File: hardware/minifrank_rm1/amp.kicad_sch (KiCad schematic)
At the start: 20 parts, among them U5 LM358

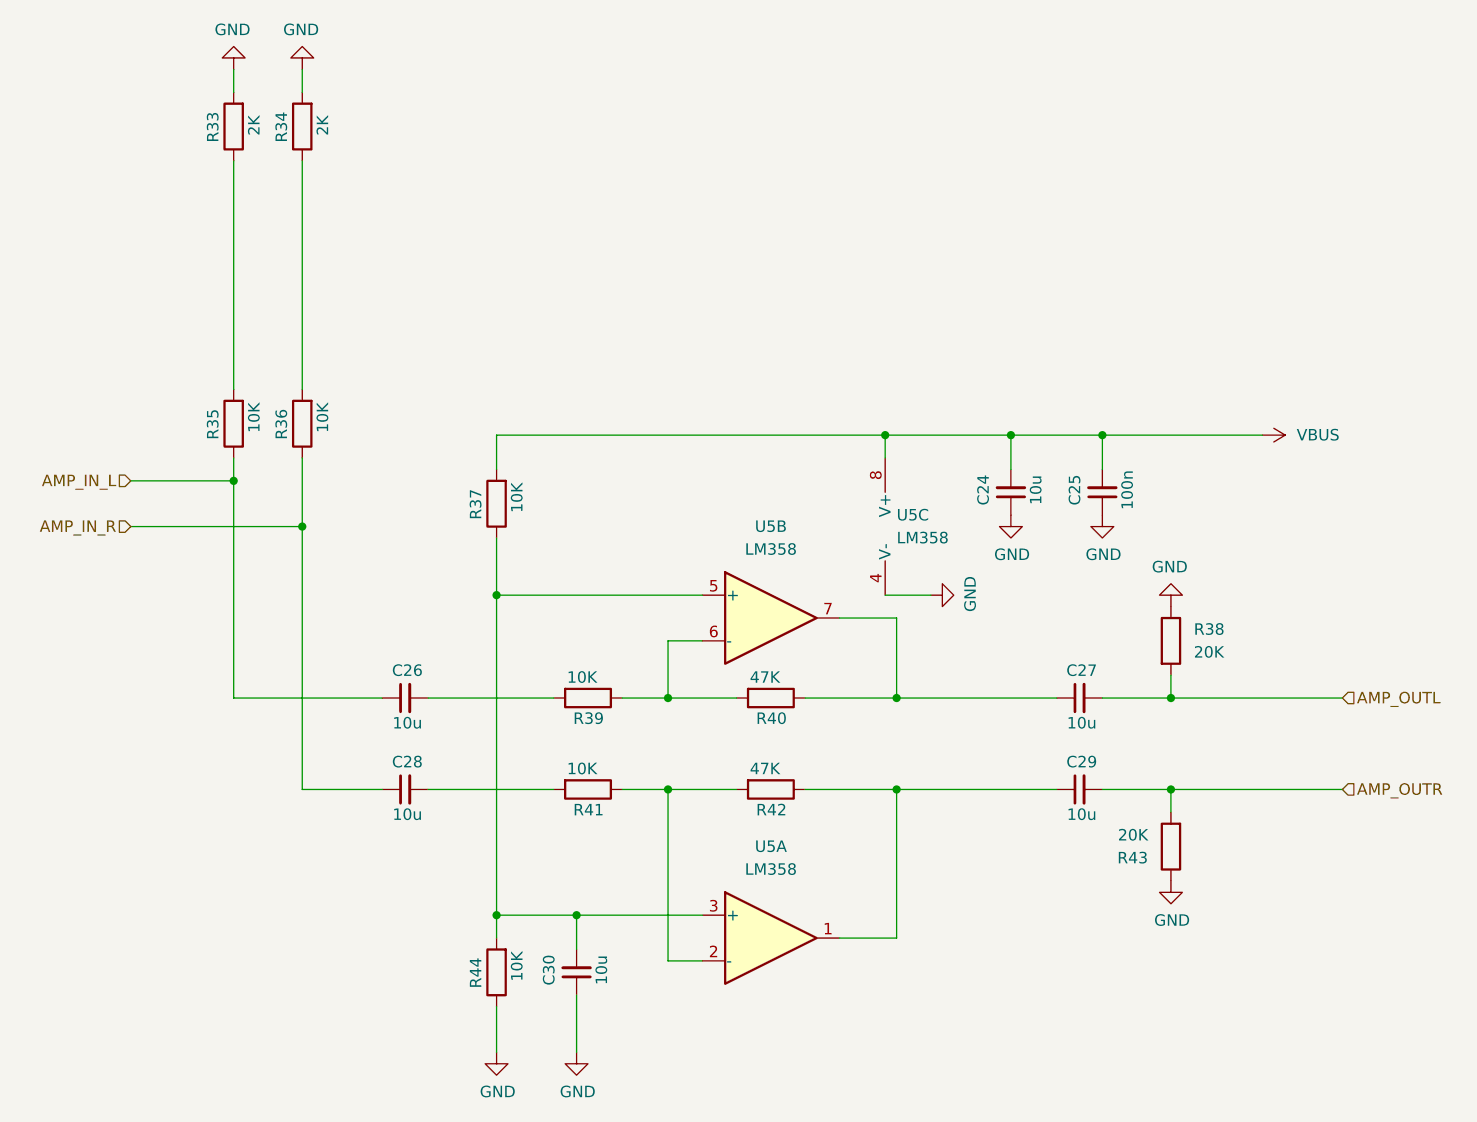
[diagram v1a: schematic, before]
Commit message: MiniFRANK 2.05 Release
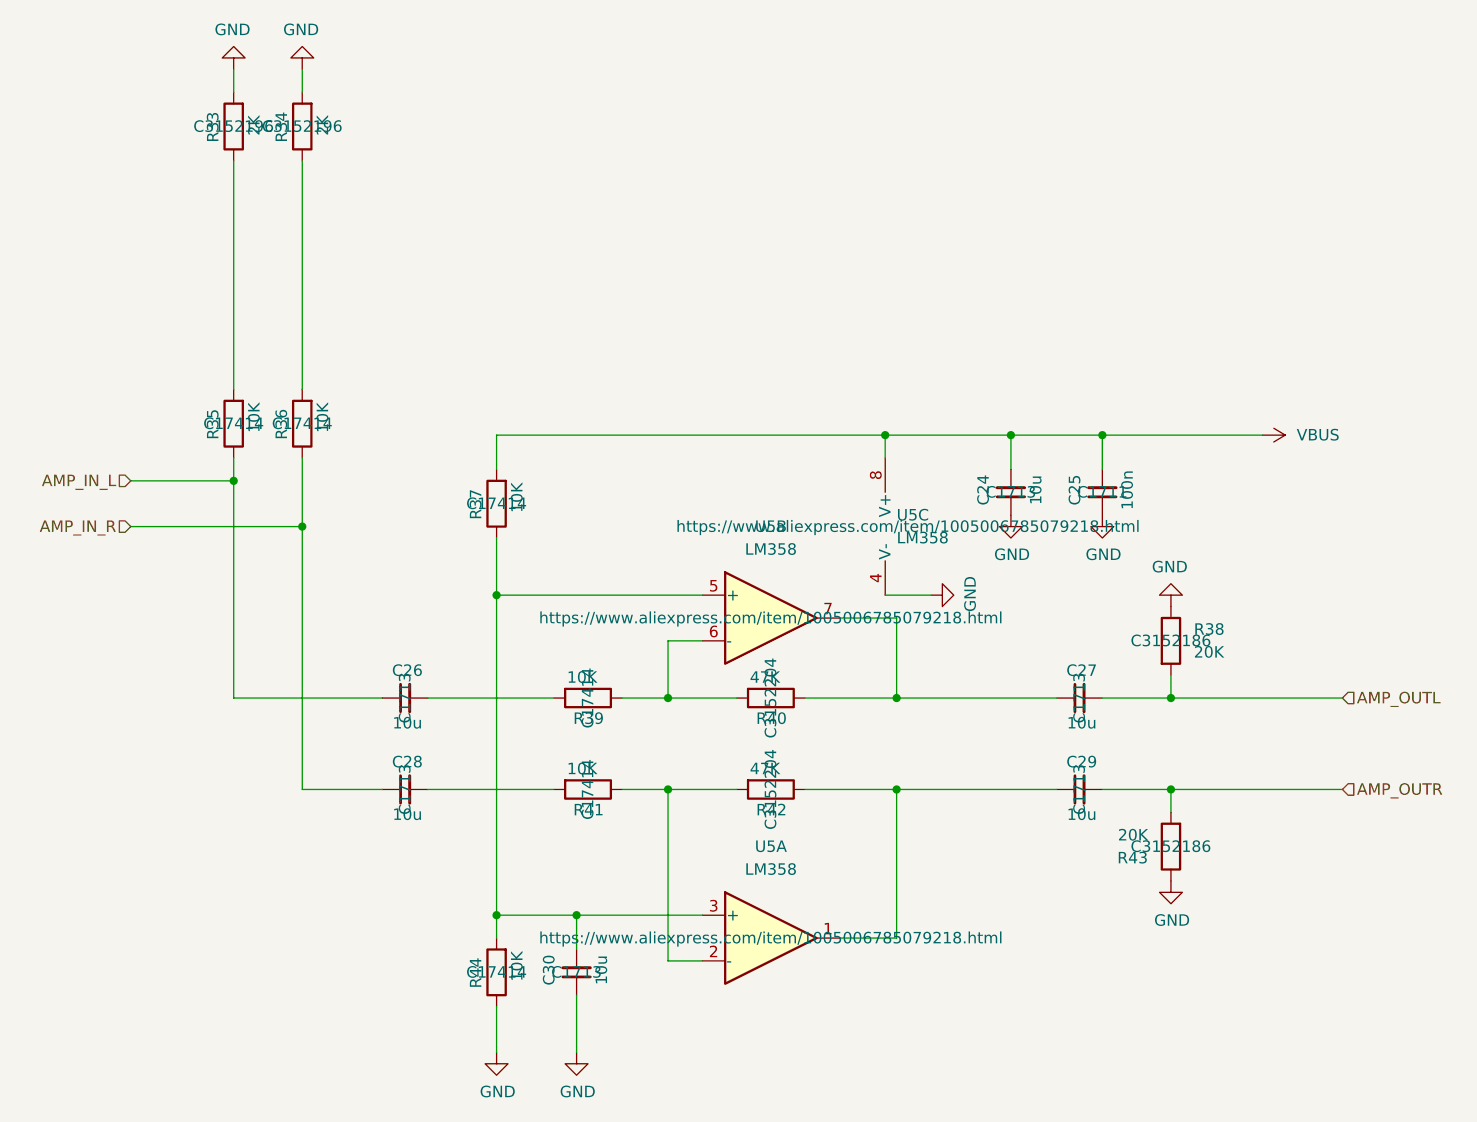
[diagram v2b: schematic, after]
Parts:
- C24, C26, C27, C28, C29, C30: LCSC (none) -> C1713
- C25: LCSC (none) -> C1711
- R33, R34: LCSC (none) -> C3152196
- R35, R36, R37, R39, R41, R44: LCSC (none) -> C17414
- R38, R43: LCSC (none) -> C3152186
- R40, R42: LCSC (none) -> C3152204
- U5: AliExpress (none) -> https://www.aliexpress.com/item/1005006785079218.html
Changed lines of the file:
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@@
 	(title_block
 		(title "MiniFRANK RM1")
-		(date "2025-04-04")
-		(rev "2.04")
+		(date "2025-04-07")
+		(rev "${VERSION}")
 		(company "Mikhail Matveev")
 		(comment 1 "https://github.com/xtremespb/frank")
@@
 			)
 		)
+		(property "LCSC" "C3152186"
+			(at 199.39 129.54 0)
+			(effects
+				(font
+					(size 1.27 1.27)
+				)
+			)
+		)
 		(pin "1"
 		)
@@
 			)
 		)
-		(property "Datasheet" "~"
+		(property "Datasheet" "https://eu.mouser.com/datasheet/2/40/KGM_X7R-3223212.pdf"
 			(at 189.23 113.03 0)
 			(effects
@@
 				)
 				(hide yes)
+			)
+		)
+		(property "LCSC" "C1713"
+			(at 189.23 113.03 0)
+			(effects
+				(font
+					(size 1.27 1.27)
+				)
 			)
 		)
@@
 			)
 		)
+		(property "LCSC" "C17414"
+			(at 102.87 82.55 0)
+			(effects
+				(font
+					(size 1.27 1.27)
+				)
+			)
+		)
 		(pin "1"
 		)
@@
 			)
 		)
+		(property "LCSC" "C17414"
+			(at 134.62 113.03 0)
+			(effects
+				(font
+					(size 1.27 1.27)
+				)
+			)
+		)
 		(pin "1"
 		)
@@
 			)
 		)
+		(property "LCSC" "C3152196"
+			(at 95.25 49.53 0)
+			(effects
+				(font
+					(size 1.27 1.27)
+				)
+			)
+		)
 		(pin "1"
 		)
@@
 			)
 		)
+		(property "LCSC" "C3152204"
+			(at 154.94 113.03 0)
+			(effects
+				(font
+					(size 1.27 1.27)
+				)
+			)
+		)
 		(pin "1"
 		)
@@
 			)
 		)
+		(property "AliExpress" "https://www.aliexpress.com/item/1005006785079218.html"
+			(at 170.18 93.98 0)
+			(effects
+				(font
+					(size 1.27 1.27)
+				)
+			)
+		)
 		(pin "6"
 		)
@@
 			)
 		)
-		(property "Datasheet" "~"
+		(property "Datasheet" "https://eu.mouser.com/datasheet/2/40/KGM_X7R-3223212.pdf"
 			(at 114.3 123.19 0)
 			(effects
@@
 				)
 				(hide yes)
+			)
+		)
+		(property "LCSC" "C1713"
+			(at 114.3 123.19 0)
+			(effects
+				(font
+					(size 1.27 1.27)
+				)
 			)
 		)
@@
 			)
 		)
+		(property "AliExpress" "https://www.aliexpress.com/item/1005006785079218.html"
+			(at 154.94 104.14 0)
+			(effects
+				(font
+					(size 1.27 1.27)
+				)
+			)
+		)
 		(pin "6"
 		)
@@
 			)
 		)
-		(property "Datasheet" "~"
+		(property "Datasheet" "https://eu.mouser.com/datasheet/2/40/KGM_X7R-3223212.pdf"
 			(at 189.23 123.19 0)
 			(effects
@@
 				)
 				(hide yes)
+			)
+		)
+		(property "LCSC" "C1713"
+			(at 189.23 123.19 0)
+			(effects
+				(font
+					(size 1.27 1.27)
+				)
 			)
 		)
@@
 			)
 		)
-		(property "Datasheet" "~"
+		(property "Datasheet" "https://eu.mouser.com/datasheet/2/40/KGM_X7R-3223212.pdf"
 			(at 133.35 143.51 0)
 			(effects
@@
 				)
 				(hide yes)
+			)
+		)
+		(property "LCSC" "C1713"
+			(at 133.35 143.51 0)
+			(effects
+				(font
+					(size 1.27 1.27)
+				)
 			)
 		)
@@
 			)
 		)
+		(property "LCSC" "C17414"
+			(at 124.46 143.51 0)
+			(effects
+				(font
+					(size 1.27 1.27)
+				)
+			)
+		)
 		(pin "1"
 		)
@@
 			)
 		)
+		(property "LCSC" "C3152204"
+			(at 154.94 123.19 0)
+			(effects
+				(font
+					(size 1.27 1.27)
+				)
+			)
+		)
 		(pin "1"
 		)
@@
 			)
 		)
+		(property "LCSC" "C17414"
+			(at 134.62 123.19 0)
+			(effects
+				(font
+					(size 1.27 1.27)
+				)
+			)
+		)
 		(pin "1"
 		)
@@
 			)
 		)
+		(property "AliExpress" "https://www.aliexpress.com/item/1005006785079218.html"
+			(at 154.94 139.7 0)
+			(effects
+				(font
+					(size 1.27 1.27)
+				)
+			)
+		)
 		(pin "6"
 		)
@@
 			)
 		)
+		(property "LCSC" "C3152186"
+			(at 199.39 106.68 0)
+			(effects
+				(font
+					(size 1.27 1.27)
+				)
+			)
+		)
 		(pin "1"
 		)
@@
 			)
 		)
+		(property "LCSC" "C17414"
+			(at 95.25 82.55 0)
+			(effects
+				(font
+					(size 1.27 1.27)
+				)
+			)
+		)
 		(pin "1"
 		)
@@
 			)
 		)
-		(property "Datasheet" "~"
+		(property "Datasheet" "https://eu.mouser.com/datasheet/2/40/KGM_X7R-3223212.pdf"
 			(at 191.77 90.17 0)
 			(effects
@@
 				)
 				(hide yes)
+			)
+		)
+		(property "LCSC" "C1711"
+			(at 191.77 90.17 0)
+			(effects
+				(font
+					(size 1.27 1.27)
+				)
 			)
 		)
@@
 			)
 		)
-		(property "Datasheet" "~"
+		(property "Datasheet" "https://eu.mouser.com/datasheet/2/40/KGM_X7R-3223212.pdf"
 			(at 114.3 113.03 0)
 			(effects
@@
 				)
 				(hide yes)
+			)
+		)
+		(property "LCSC" "C1713"
+			(at 114.3 113.03 0)
+			(effects
+				(font
+					(size 1.27 1.27)
+				)
 			)
 		)
@@
 			)
 		)
+		(property "LCSC" "C17414"
+			(at 124.46 91.44 0)
+			(effects
+				(font
+					(size 1.27 1.27)
+				)
+			)
+		)
 		(pin "1"
 		)
@@
 			)
 		)
-		(property "Datasheet" "~"
+		(property "Datasheet" "https://eu.mouser.com/datasheet/2/40/KGM_X7R-3223212.pdf"
 			(at 181.61 90.17 0)
 			(effects
@@
 				)
 				(hide yes)
+			)
+		)
+		(property "LCSC" "C1713"
+			(at 181.61 90.17 0)
+			(effects
+				(font
+					(size 1.27 1.27)
+				)
 			)
 		)
@@
 			)
 		)
+		(property "LCSC" "C3152196"
+			(at 102.87 49.53 0)
+			(effects
+				(font
+					(size 1.27 1.27)
+				)
+			)
+		)
